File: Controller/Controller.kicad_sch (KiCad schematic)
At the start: 16 parts, among them U35 LMK1C1103 PW, Y3 ECS-3225MV-250-CN

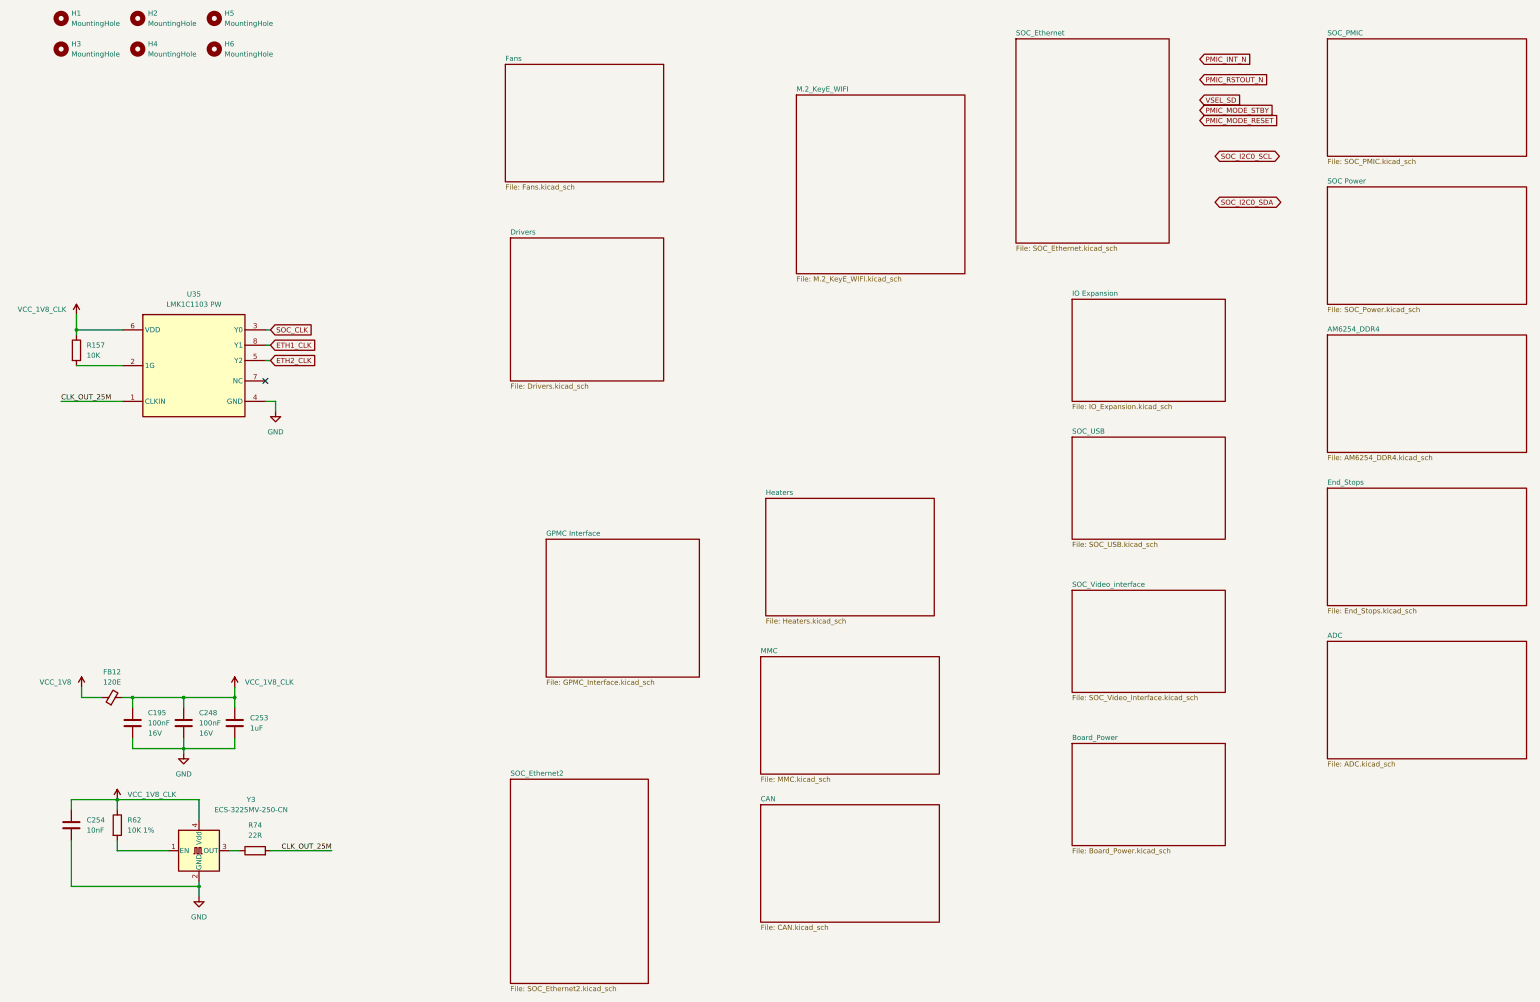
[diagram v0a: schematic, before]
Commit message: Fixed some minor issues, started some scheamtic clean up
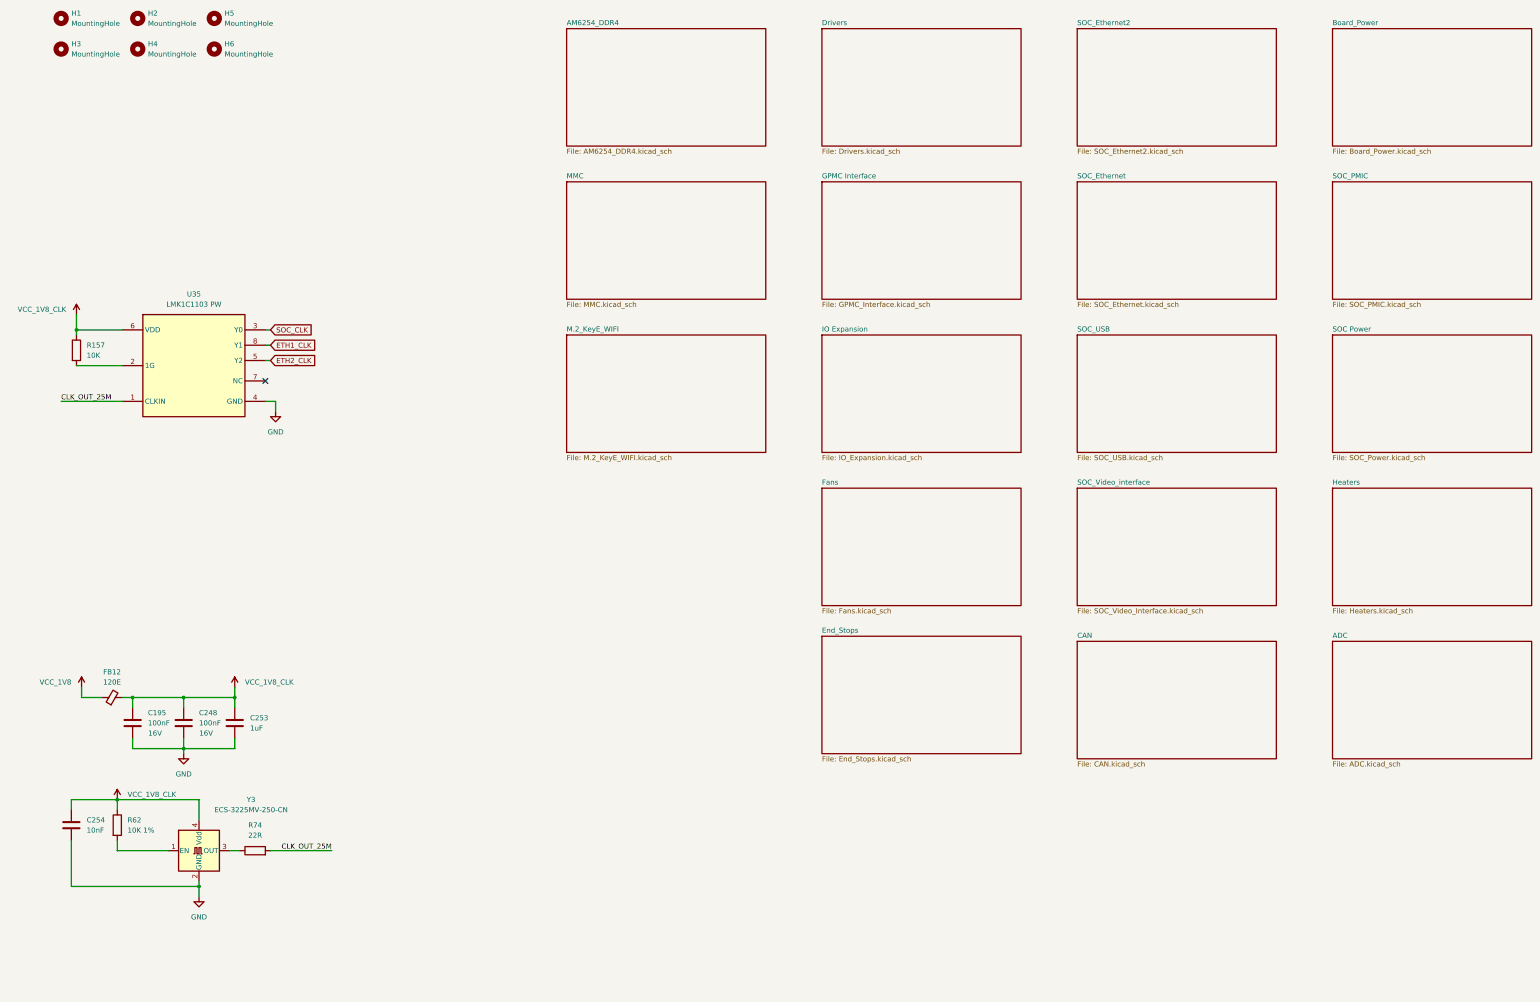
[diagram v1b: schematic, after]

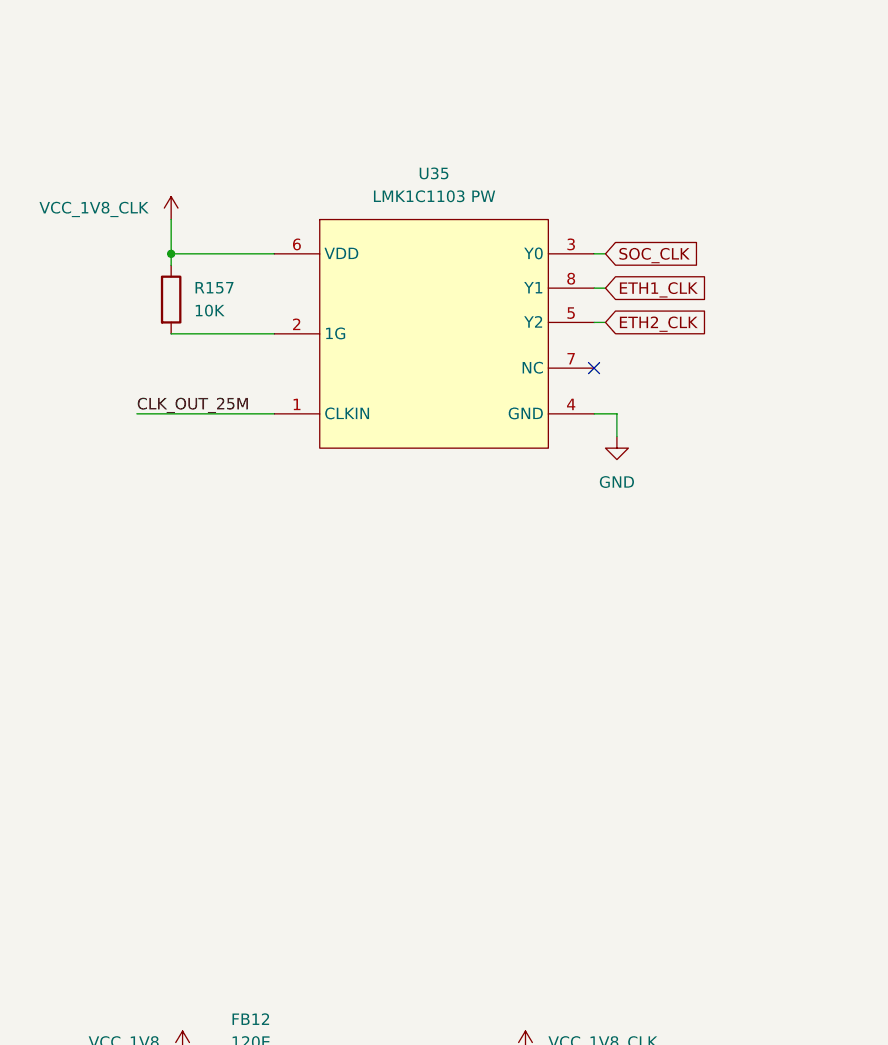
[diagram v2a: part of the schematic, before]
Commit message: Testpoints + DDR velocity comp
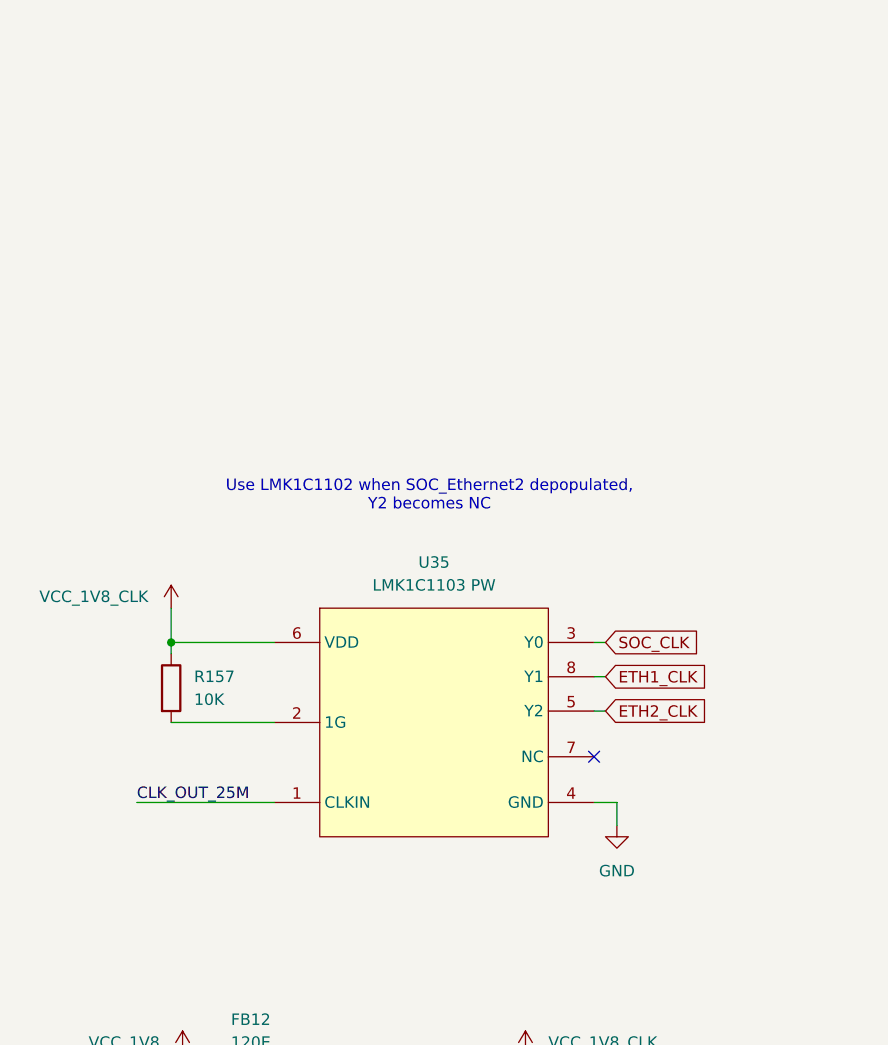
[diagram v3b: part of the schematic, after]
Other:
- note added: "Use LMK1C1102 when SOC_Ethernet2 depopulated, Y2 becomes NC"
- moved on the sheet: R157, U35
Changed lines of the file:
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@@
 	(generator_version "10.0")
 	(paper "A3")
+	(text "Use LMK1C1102 when SOC_Ethernet2 depopulated,\nY2 becomes NC"
+		(exclude_from_sim no)
+		(at 60.452 127.254 0)
+		(effects
+			(font
+				(size 1.27 1.27)
+			)
+		)
+	)
 	(junction
 		(at 58.42 191.77)
@@
 	)
 	(junction
-		(at 31.75 100.33)
+		(at 31.75 143.51)
 		(diameter 0)
 		(color 0 0 0 0)
@@
 	)
 	(no_connect
-		(at 78.74 113.03)
-	)
-	(wire
-		(pts
-			(xy 31.75 96.52) (xy 31.75 100.33)
-		)
-		(stroke
-			(width 0)
-			(type default)
-		)
-	)
-	(wire
-		(pts
-			(xy 31.75 100.33) (xy 43.18 100.33)
+		(at 78.74 156.21)
+	)
+	(wire
+		(pts
+			(xy 31.75 139.7) (xy 31.75 143.51)
+		)
+		(stroke
+			(width 0)
+			(type default)
+		)
+	)
+	(wire
+		(pts
+			(xy 31.75 143.51) (xy 43.18 143.51)
 		)
 		(stroke
@@
 	(wire
 		(pts
-			(xy 80.01 100.33) (xy 78.74 100.33)
+			(xy 80.01 143.51) (xy 78.74 143.51)
 		)
 		(stroke
@@
 	(wire
 		(pts
-			(xy 80.01 104.14) (xy 78.74 104.14)
+			(xy 80.01 147.32) (xy 78.74 147.32)
 		)
 		(stroke
@@
 	(wire
 		(pts
-			(xy 31.75 101.6) (xy 31.75 100.33)
+			(xy 31.75 144.78) (xy 31.75 143.51)
 		)
 		(stroke
@@
 	(wire
 		(pts
-			(xy 81.28 120.65) (xy 81.28 118.11)
+			(xy 81.28 163.83) (xy 81.28 161.29)
 		)
 		(stroke
@@
 	(wire
 		(pts
-			(xy 80.01 107.95) (xy 78.74 107.95)
-		)
-		(stroke
-			(width 0)
-			(type default)
-		)
-	)
-	(wire
-		(pts
-			(xy 43.18 118.11) (xy 27.94 118.11)
+			(xy 80.01 151.13) (xy 78.74 151.13)
+		)
+		(stroke
+			(width 0)
+			(type default)
+		)
+	)
+	(wire
+		(pts
+			(xy 43.18 161.29) (xy 27.94 161.29)
 		)
 		(stroke
@@
 	(wire
 		(pts
-			(xy 81.28 118.11) (xy 78.74 118.11)
+			(xy 81.28 161.29) (xy 78.74 161.29)
 		)
 		(stroke
@@
 	(wire
 		(pts
-			(xy 31.75 109.22) (xy 43.18 109.22)
+			(xy 31.75 152.4) (xy 43.18 152.4)
 		)
 		(stroke
@@
 	)
 	(label "CLK_OUT_25M"
-		(at 27.94 118.11 0)
+		(at 27.94 161.29 0)
 		(effects
 			(font
@@
 	(global_label "ETH1_CLK"
 		(shape input)
-		(at 80.01 104.14 0)
+		(at 80.01 147.32 0)
 		(fields_autoplaced yes)
 		(effects
@@
 		)
 		(property "Intersheetrefs" "${INTERSHEET_REFS}"
-			(at 92.1875 104.14 0)
+			(at 92.1875 147.32 0)
 			(hide yes)
 			(show_name no)
@@
 	(global_label "SOC_CLK"
 		(shape input)
-		(at 80.01 100.33 0)
+		(at 80.01 143.51 0)
 		(fields_autoplaced yes)
 		(effects
@@
 		)
 		(property "Intersheetrefs" "${INTERSHEET_REFS}"
-			(at 91.3409 100.33 0)
+			(at 91.3409 143.51 0)
 			(hide yes)
 			(show_name no)
@@
 	(global_label "ETH2_CLK"
 		(shape input)
-		(at 80.01 107.95 0)
+		(at 80.01 151.13 0)
 		(fields_autoplaced yes)
 		(effects
@@
 		)
 		(property "Intersheetrefs" "${INTERSHEET_REFS}"
-			(at 92.1875 107.95 0)
+			(at 92.1875 151.13 0)
 			(hide yes)
 			(show_name no)
@@
 	(symbol
 		(lib_id "IC:LMK1C1103")
-		(at 60.96 109.22 0)
+		(at 60.96 152.4 0)
 		(unit 1)
 		(body_style 1)
@@
 		(fields_autoplaced yes)
 		(property "Reference" "U35"
-			(at 60.96 91.44 0)
+			(at 60.96 134.62 0)
 			(show_name no)
 			(do_not_autoplace no)
@@
 		)
 		(property "Value" "LMK1C1103 PW"
-			(at 60.96 93.98 0)
+			(at 60.96 137.16 0)
 			(show_name no)
 			(do_not_autoplace no)
@@
 		)
 		(property "Footprint" "Libs:LMK1C110X TSSOP-8"
-			(at 60.96 109.22 0)
+			(at 60.96 152.4 0)
 			(hide yes)
 			(show_name no)
@@
 		)
 		(property "Datasheet" ""
-			(at 60.96 109.22 0)
+			(at 60.96 152.4 0)
 			(hide yes)
 			(show_name no)
@@
 		)
 		(property "Description" ""
-			(at 60.96 109.22 0)
+			(at 60.96 152.4 0)
 			(hide yes)
 			(show_name no)
@@
 	(symbol
 		(lib_id "power:VCC")
-		(at 31.75 96.52 0)
+		(at 31.75 139.7 0)
 		(mirror y)
 		(unit 1)
@@
 		(dnp no)
 		(property "Reference" "#PWR0371"
-			(at 31.75 100.33 0)
+			(at 31.75 143.51 0)
 			(hide yes)
 			(show_name no)
@@
 		)
 		(property "Value" "VCC_1V8_CLK"
-			(at 29.21 95.2499 0)
+			(at 29.21 138.4299 0)
 			(show_name no)
 			(do_not_autoplace no)
@@
 		)
 		(property "Footprint" ""
-			(at 31.75 96.52 0)
+			(at 31.75 139.7 0)
 			(hide yes)
 			(show_name no)
@@
 		)
 		(property "Datasheet" ""
-			(at 31.75 96.52 0)
+			(at 31.75 139.7 0)
 			(hide yes)
 			(show_name no)
@@
 		)
 		(property "Description" "Power symbol creates a global label with name \"VCC\""
-			(at 31.75 96.52 0)
+			(at 31.75 139.7 0)
 			(hide yes)
 			(show_name no)
@@
 	(symbol
 		(lib_id "power:GND")
-		(at 81.28 120.65 0)
+		(at 81.28 163.83 0)
 		(unit 1)
 		(body_style 1)
@@
 		(fields_autoplaced yes)
 		(property "Reference" "#PWR0372"
-			(at 81.28 127 0)
+			(at 81.28 170.18 0)
 			(hide yes)
 			(show_name no)
@@
 		)
 		(property "Value" "GND"
-			(at 81.28 125.73 0)
+			(at 81.28 168.91 0)
 			(show_name no)
 			(do_not_autoplace no)
@@
 		)
 		(property "Footprint" ""
-			(at 81.28 120.65 0)
+			(at 81.28 163.83 0)
 			(hide yes)
 			(show_name no)
@@
 		)
 		(property "Datasheet" ""
-			(at 81.28 120.65 0)
+			(at 81.28 163.83 0)
 			(hide yes)
 			(show_name no)
@@
 		)
 		(property "Description" "Power symbol creates a global label with name \"GND\" , ground"
-			(at 81.28 120.65 0)
+			(at 81.28 163.83 0)
 			(hide yes)
 			(show_name no)
@@
 	(symbol
 		(lib_id "Device:R")
-		(at 31.75 105.41 0)
+		(at 31.75 148.59 0)
 		(unit 1)
 		(body_style 1)
@@
 		(fields_autoplaced yes)
 		(property "Reference" "R157"
-			(at 34.29 104.1399 0)
+			(at 34.29 147.3199 0)
 			(show_name no)
 			(do_not_autoplace no)
@@
 		)
 		(property "Value" "10K"
-			(at 34.29 106.6799 0)
+			(at 34.29 149.8599 0)
 			(show_name no)
 			(do_not_autoplace no)
@@
 		)
 		(property "Footprint" "Resistor_SMD:R_0603_1608Metric"
-			(at 29.972 105.41 90)
+			(at 29.972 148.59 90)
 			(hide yes)
 			(show_name no)
@@
 		)
 		(property "Datasheet" ""
-			(at 31.75 105.41 0)
+			(at 31.75 148.59 0)
 			(hide yes)
 			(show_name no)
@@
 		)
 		(property "Description" "Resistor"
-			(at 31.75 105.41 0)
-			(hide yes)
-			(show_name no)
+			(at 31.75 148.59 0)
+			(hide yes)
+			(show_name no)
